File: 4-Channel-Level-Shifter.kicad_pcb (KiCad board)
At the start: 2 copper layers, 16.5 x 18.2 mm, 16 parts, among them J1 5V side, J2 3.3V side, Q1 BSS138, Q2 BSS138, Q3 BSS138, Q4 BSS138

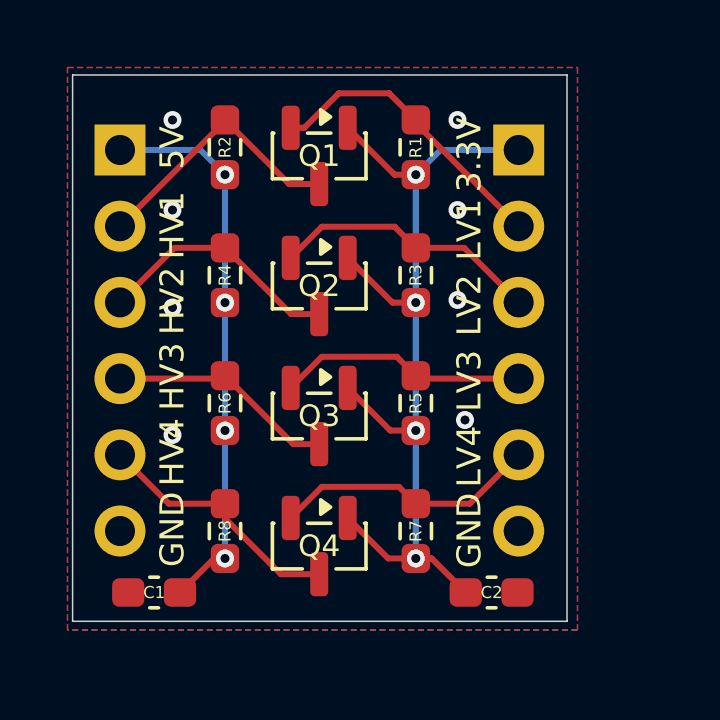
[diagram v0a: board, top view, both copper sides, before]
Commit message: Update schematic
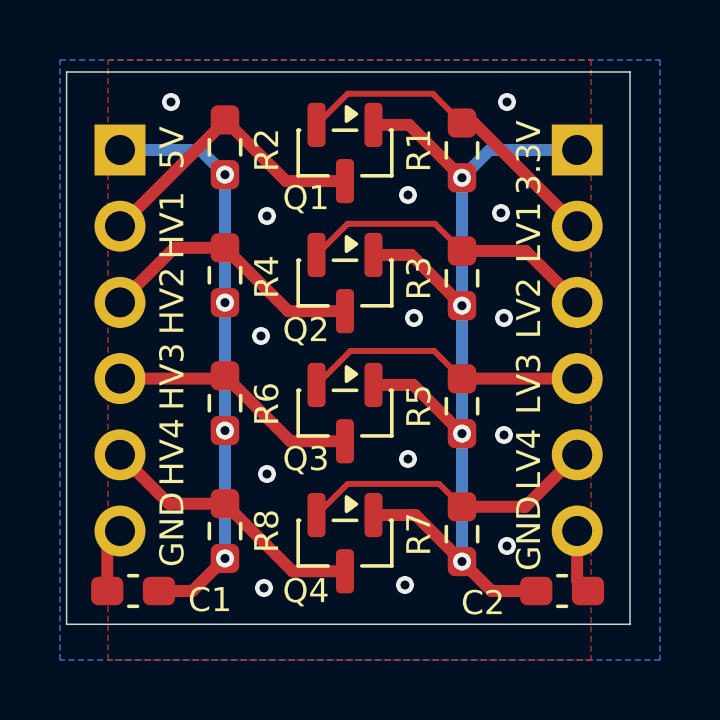
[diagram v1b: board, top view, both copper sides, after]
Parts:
- moved C2 2.35 mm to (64.7, 64.7)
- moved J2 1.95 mm to (65.2, 50.0)
- moved R1 1.54 mm to (61.4, 50.0)
- moved R3 1.54 mm to (61.4, 54.3)
- moved R5 1.54 mm to (61.4, 58.5)
- moved R7 1.54 mm to (61.4, 62.8)
- moved Q4 0.87 mm to (57.5, 63.1)
- moved Q1 0.87 mm to (57.5, 50.1)
- moved Q2 0.87 mm to (57.5, 54.4)
- moved Q3 0.87 mm to (57.5, 58.8)
- moved C1 0.70 mm to (50.4, 64.7)
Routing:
- net GND: track 0.00 -> 4.33 mm, vias 8 -> 14
- net +3.3V: track 30.2 -> 34.4 mm
- net /LV3: track 8.33 -> 9.55 mm
- net /LV4: track 8.94 -> 10.2 mm
- net /LV2: track 9.07 -> 10.2 mm
- net +5V: track 18.6 -> 19.6 mm
- net /LV1: track 9.98 -> 10.9 mm
- net /HV1: track 9.02 -> 9.84 mm
- net /HV3: track 7.62 -> 8.44 mm
- net /HV2: track 8.31 -> 9.13 mm
- net /HV4: track 8.57 -> 9.11 mm
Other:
- board size 16.5 x 18.2 mm -> 18.8 x 18.4 mm
